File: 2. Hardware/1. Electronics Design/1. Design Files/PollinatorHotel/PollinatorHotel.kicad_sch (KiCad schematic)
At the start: 10 parts, among them J1 Conn_01x02_Socket, SW1 SW_Push, U1 DHT11, U2 DHT11, U3 DHT11

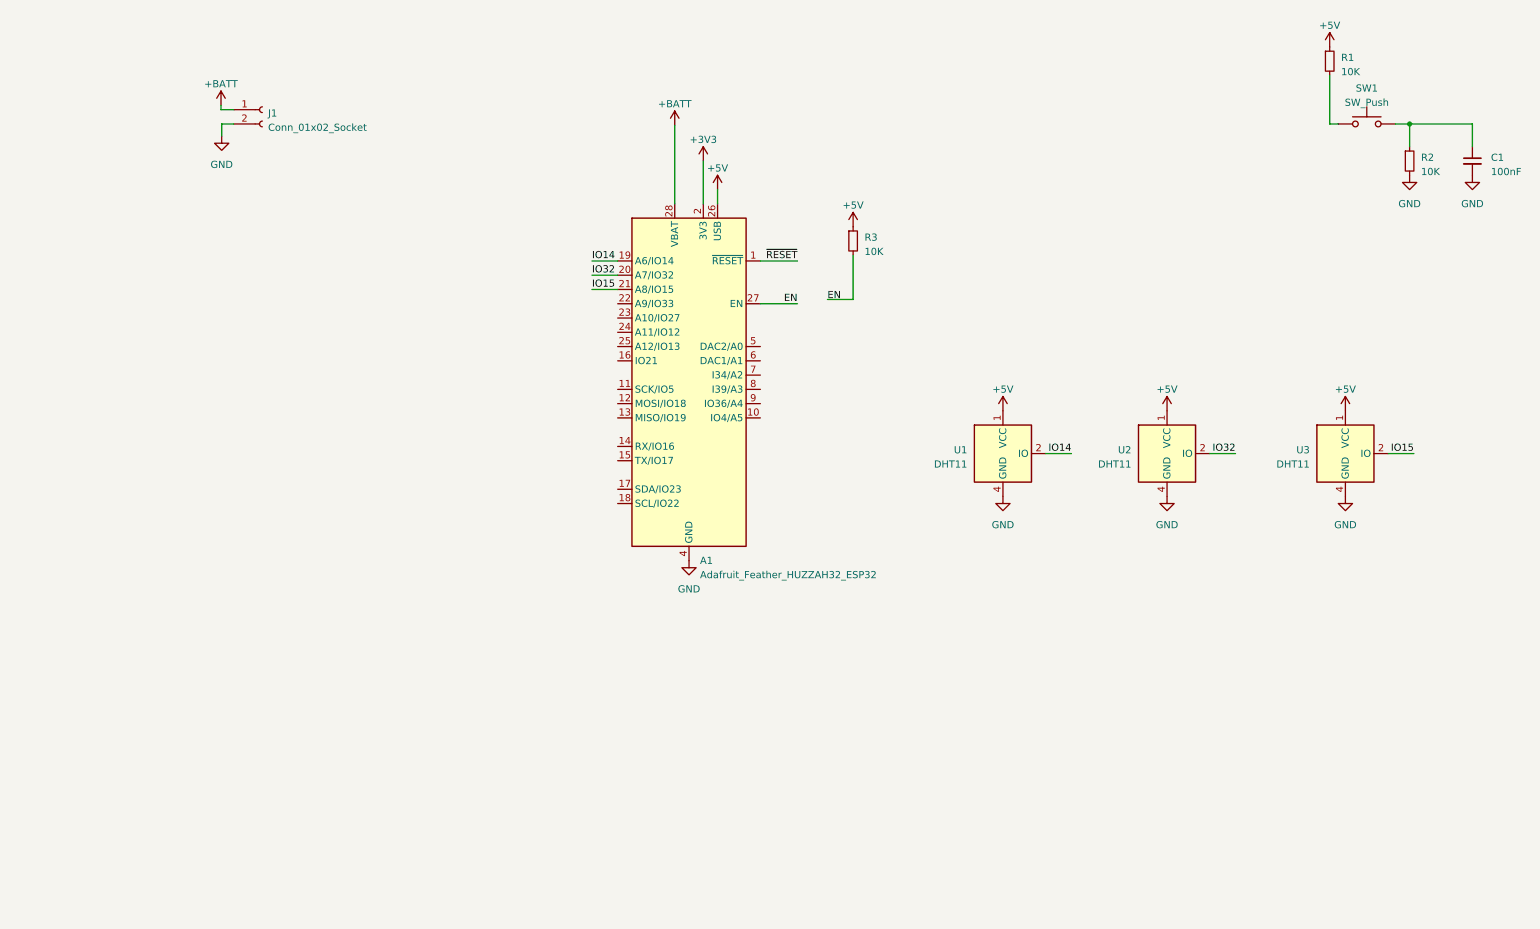
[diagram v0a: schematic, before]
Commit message: Updated Schematic
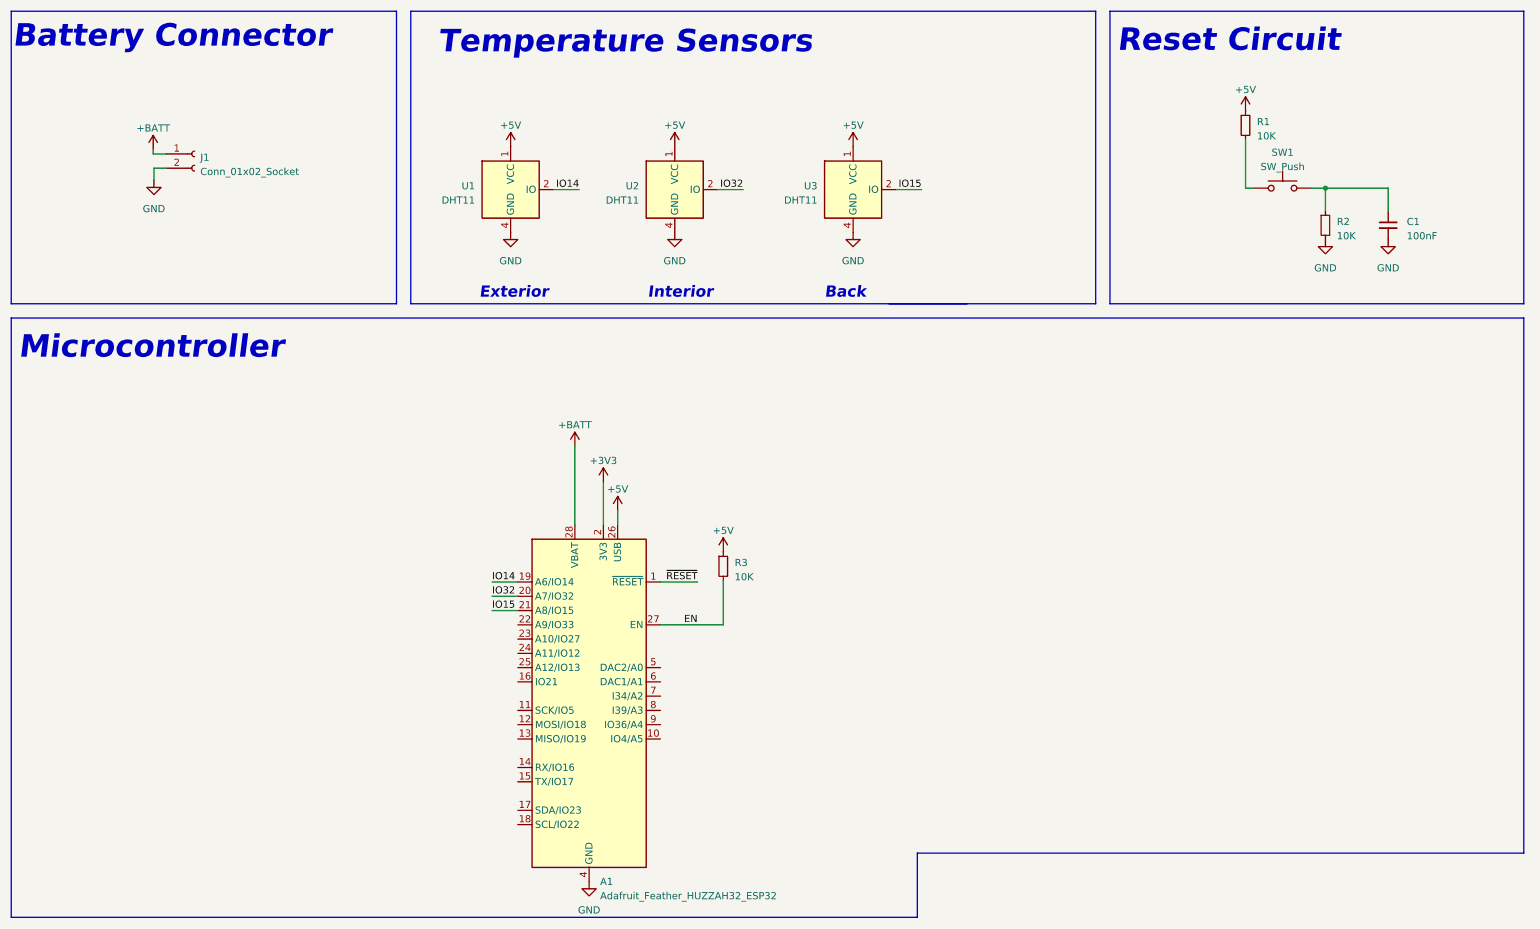
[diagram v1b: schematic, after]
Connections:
- net EN: now also R3.2
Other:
- note added: "Back"
- note added: "Battery Connector"
- note added: "Exterior"
- note added: "Interior"
- note added: "Microcontroller"
- note added: "Reset Circuit"
- note added: "Temperature Sensors"
- moved on the sheet: A1, C1, J1, R1, R2, R3, SW1, U1, U2, U3
